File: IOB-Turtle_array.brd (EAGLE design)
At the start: 106.7 x 104.1 mm, 92 parts

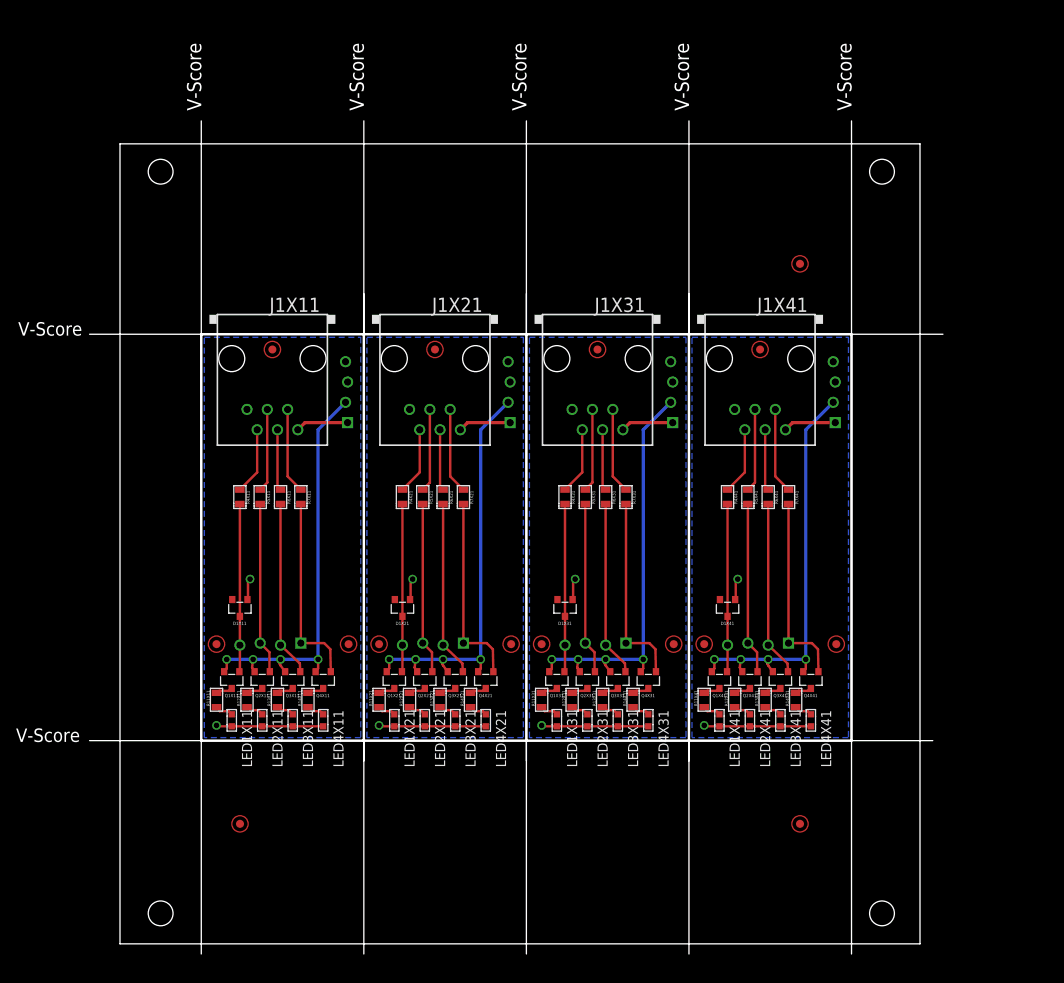
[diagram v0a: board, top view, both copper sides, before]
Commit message: Version 2.0
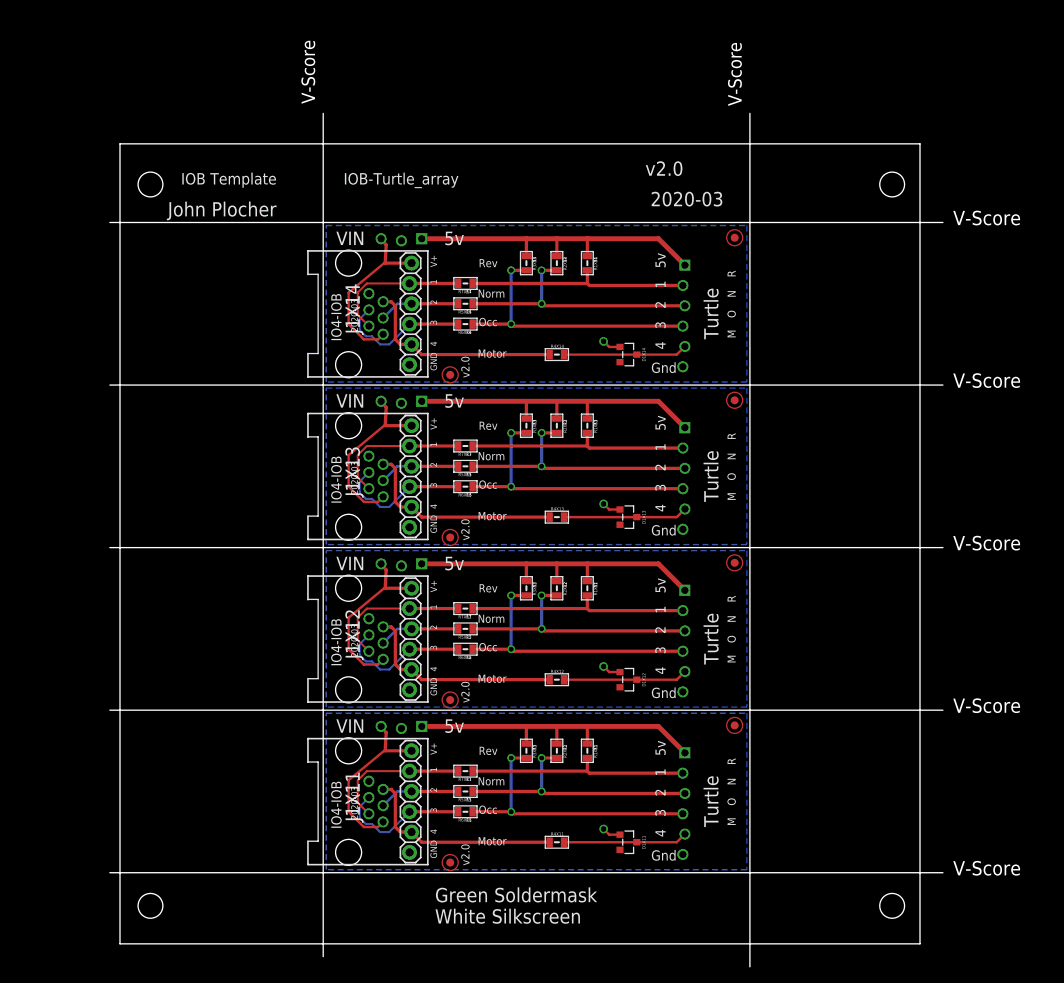
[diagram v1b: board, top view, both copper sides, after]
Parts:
- removed D1X21, D1X31, D1X41, Q1X11, Q1X21, Q1X31, Q1X41, Q2X11, Q2X21, Q2X31, Q2X41, Q3X11, Q3X21, Q3X31, Q3X41, Q4X11, Q4X21, Q4X31, Q4X41: (no value), SPCoast:SOT23-3
- removed FID1X21, FID1X31, FID1X41, FID2X21, FID2X31, FID2X41, FID3X11, FID3X21, FID3X31, FID3X41, R8X2, R8X3, R8X4: (no value), SPCoast:FIDUCIAL_1MM
- removed IOBX11, IOBX21, IOBX31, IOBX41: (no value), SPCoast:IO4-IOB
- removed J1X21, J1X31, J1X41: (no value), SPCoast:RJ25
- removed LED1X11, LED1X21, LED1X31, LED1X41, LED2X11, LED2X21, LED2X31, LED2X41, LED3X11, LED3X21, LED3X31, LED3X41, LED4X11, LED4X21, LED4X31, LED4X41: (no value), SPCoast:0603-LED
- removed R11X11, R11X21, R11X31, R11X41, R12X11, R12X21, R12X31, R12X41, R13X11, R13X21, R13X31, R13X41, R14X11, R14X21, R14X31, R14X41, R4X21, R4X31, R4X41, R5X21, R5X31, R5X41, R6X21, R6X31, R6X41, R7X21, R7X31, R7X41: (no value), SPCoast:0805-RES
- removed R8X1: (no value), SPCoast:BOARD-DINRAIL-3.17IN-4X-IOB
- added D1X12, D1X13, D1X14: (no value), SPCoast:SOT23-3
- added FID1X12, FID1X13, FID1X14, FID2X12, FID2X13, FID2X14: (no value), SPCoast:FIDUCIAL_1MM
- added J1X12, J1X13, J1X14: (no value), SPCoast:RJ24-INVERTED-PINS
- added R1X11, R1X12, R1X13, R1X14, R2X11, R2X12, R2X13, R2X14, R3X11, R3X12, R3X13, R3X14, R4X12, R4X13, R4X14, R5X12, R5X13, R5X14, R6X12, R6X13, R6X14, R7X12, R7X13, R7X14: (no value), SPCoast:0805-RES
- added U$1X1: (no value), SPCoast:BOARD-DINRAIL-3.17IN-H4X-IOB
- added U$1X11, U$1X12, U$1X13, U$1X14: (no value), SPCoast:IO4-IOB
- J1X11: device SPCoast:RJ25 -> SPCoast:RJ24-INVERTED-PINS
- moved FID1X11 67.9 mm to (41.3, 10.2), turned to 0 degrees
- moved FID2X11 65.6 mm to (76.8, 27.3), turned to 0 degrees
- moved R4X11 58.6 mm to (54.6, 12.7), turned to 0 degrees
- moved J1X11 57.0 mm to (32.4, 17.8), turned to 90 degrees
- moved D1X11 56.7 mm to (63.5, 12.7), turned to 270 degrees
- moved R6X11 45.7 mm to (43.2, 16.5), turned to 180 degrees
- moved R5X11 44.9 mm to (43.2, 19.1), turned to 180 degrees
- moved R7X11 40.0 mm to (43.2, 21.6), turned to 180 degrees
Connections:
- removed net !KTX11: J1X11.5, R4X11.1
- removed net !KTX21: J1X21.5, R4X21.1
- removed net !KTX31: J1X31.5, R4X31.1
- removed net !KTX41: J1X41.5, R4X41.1
- removed net !NORMX21: J1X21.3, R6X21.1
- removed net !NORMX31: J1X31.3, R6X31.1
- removed net !NORMX41: J1X41.3, R6X41.1
- removed net !OCCX21: J1X21.4, R5X21.1
- removed net !OCCX31: J1X31.4, R5X31.1
- removed net !OCCX41: J1X41.4, R5X41.1
- removed net !REVX21: J1X21.2, R7X21.1
- removed net !REVX31: J1X31.2, R7X31.1
- removed net !REVX41: J1X41.2, R7X41.1
- removed net GNDX21: D1X21.1, IOBX21.G@1, IOBX21.G@2, J1X21.6, LED1X21.C, LED2X21.C, LED3X21.C, LED4X21.C
- removed net GNDX31: D1X31.1, IOBX31.G@1, IOBX31.G@2, J1X31.6, LED1X31.C, LED2X31.C, LED3X31.C, LED4X31.C
- removed net GNDX41: D1X41.1, IOBX41.G@1, IOBX41.G@2, J1X41.6, LED1X41.C, LED2X41.C, LED3X41.C, LED4X41.C
- removed net N$11X11: Q4X11.3, R14X11.2
- removed net N$11X21: Q4X21.3, R14X21.2
- removed net N$11X31: Q4X31.3, R14X31.2
- removed net N$11X41: Q4X41.3, R14X41.2
- removed net N$2X11: LED4X11.A, R14X11.1
- removed net N$2X21: LED4X21.A, R14X21.1
- removed net N$2X31: LED4X31.A, R14X31.1
- removed net N$2X41: LED4X41.A, R14X41.1
- removed net N$30X11: Q3X11.3, R13X11.2
- removed net N$30X21: Q3X21.3, R13X21.2
- removed net N$30X31: Q3X31.3, R13X31.2
- removed net N$30X41: Q3X41.3, R13X41.2
- removed net N$31X11: Q2X11.3, R12X11.2
- removed net N$31X21: Q2X21.3, R12X21.2
- removed net N$31X31: Q2X31.3, R12X31.2
- removed net N$31X41: Q2X41.3, R12X41.2
- removed net N$32X11: Q1X11.3, R11X11.2
- removed net N$32X21: Q1X21.3, R11X21.2
- removed net N$32X31: Q1X31.3, R11X31.2
- removed net N$32X41: Q1X41.3, R11X41.2
- removed net N$3X11: LED3X11.A, R13X11.1
- removed net N$3X21: LED3X21.A, R13X21.1
- removed net N$3X31: LED3X31.A, R13X31.1
- removed net N$3X41: LED3X41.A, R13X41.1
- removed net N$4X11: LED2X11.A, R12X11.1
- removed net N$4X21: LED2X21.A, R12X21.1
- removed net N$4X31: LED2X31.A, R12X31.1
- removed net N$4X41: LED2X41.A, R12X41.1
- removed net N$5X11: LED1X11.A, R11X11.1
- removed net N$5X21: LED1X21.A, R11X21.1
- removed net N$5X31: LED1X31.A, R11X31.1
- removed net N$5X41: LED1X41.A, R11X41.1
- removed net P1X11: IOBX11.P1, Q4X11.1, R7X11.2
- removed net P1X21: IOBX21.P1, Q4X21.1, R7X21.2
- removed net P1X31: IOBX31.P1, Q4X31.1, R7X31.2
- removed net P1X41: IOBX41.P1, Q4X41.1, R7X41.2
- removed net P2X11: IOBX11.P2, Q3X11.1, R6X11.2
- removed net P2X21: IOBX21.P2, Q3X21.1, R6X21.2
- removed net P2X31: IOBX31.P2, Q3X31.1, R6X31.2
- removed net P2X41: IOBX41.P2, Q3X41.1, R6X41.2
- removed net P3X11: IOBX11.P3, Q2X11.1, R5X11.2
- removed net P3X21: IOBX21.P3, Q2X21.1, R5X21.2
- removed net P3X31: IOBX31.P3, Q2X31.1, R5X31.2
- removed net P3X41: IOBX41.P3, Q2X41.1, R5X41.2
- removed net P4X21: D1X21.3, IOBX21.P4, Q1X21.1, R4X21.2
- removed net P4X31: D1X31.3, IOBX31.P4, Q1X31.1, R4X31.2
- removed net P4X41: D1X41.3, IOBX41.P4, Q1X41.1, R4X41.2
- removed net VCCIOX21: IOBX21.V+, J1X21.1
- removed net VCCIOX31: IOBX31.V+, J1X31.1
- removed net VCCIOX41: IOBX41.V+, J1X41.1
- removed net VCCX21: IOBX21.V5, Q1X21.2, Q2X21.2, Q3X21.2, Q4X21.2
- removed net VCCX31: IOBX31.V5, Q1X31.2, Q2X31.2, Q3X31.2, Q4X31.2
- removed net VCCX41: IOBX41.V5, Q1X41.2, Q2X41.2, Q3X41.2, Q4X41.2
- new net !NORMX12: R2X12.2, R5X12.1, U$1X12.P2
- new net !NORMX13: R2X13.2, R5X13.1, U$1X13.P2
- new net !NORMX14: R2X14.2, R5X14.1, U$1X14.P2
- new net !OCCX12: R3X12.2, R6X12.1, U$1X12.P3
- new net !OCCX13: R3X13.2, R6X13.1, U$1X13.P3
- new net !OCCX14: R3X14.2, R6X14.1, U$1X14.P3
- new net !REVX12: R1X12.2, R7X12.1, U$1X12.P1
- new net !REVX13: R1X13.2, R7X13.1, U$1X13.P1
- new net !REVX14: R1X14.2, R7X14.1, U$1X14.P1
- new net GNDX12: D1X12.1, J1X12.6, J1X12.6@1, U$1X12.G@3
- new net GNDX13: D1X13.1, J1X13.6, J1X13.6@1, U$1X13.G@3
- new net GNDX14: D1X14.1, J1X14.6, J1X14.6@1, U$1X14.G@3
- new net IO4-2X11: J1X11.2, J1X11.2@1, R7X11.2
- new net IO4-2X12: J1X12.2, J1X12.2@1, R7X12.2
- new net IO4-2X13: J1X13.2, J1X13.2@1, R7X13.2
- new net IO4-2X14: J1X14.2, J1X14.2@1, R7X14.2
- new net IO4-3X11: J1X11.3, J1X11.3@1, R5X11.2
- new net IO4-3X12: J1X12.3, J1X12.3@1, R5X12.2
- new net IO4-3X13: J1X13.3, J1X13.3@1, R5X13.2
- new net IO4-3X14: J1X14.3, J1X14.3@1, R5X14.2
- new net IO4-4X11: J1X11.4, J1X11.4@1, R6X11.2
- new net IO4-4X12: J1X12.4, J1X12.4@1, R6X12.2
- new net IO4-4X13: J1X13.4, J1X13.4@1, R6X13.2
- new net IO4-4X14: J1X14.4, J1X14.4@1, R6X14.2
- new net IO4-5X11: J1X11.5, J1X11.5@1, R4X11.1
- new net IO4-5X12: J1X12.5, J1X12.5@1, R4X12.1
- new net IO4-5X13: J1X13.5, J1X13.5@1, R4X13.1
- new net IO4-5X14: J1X14.5, J1X14.5@1, R4X14.1
- new net P4X12: D1X12.3, R4X12.2, U$1X12.P4
- new net P4X13: D1X13.3, R4X13.2, U$1X13.P4
- new net P4X14: D1X14.3, R4X14.2, U$1X14.P4
- new net VCCIOX12: J1X12.1, J1X12.1@1, U$1X12.V+
- new net VCCIOX13: J1X13.1, J1X13.1@1, U$1X13.V+
- new net VCCIOX14: J1X14.1, J1X14.1@1, U$1X14.V+
- new net VCCX12: R1X12.1, R2X12.1, R3X12.1, U$1X12.V5, U$1X12.V5@1
- new net VCCX13: R1X13.1, R2X13.1, R3X13.1, U$1X13.V5, U$1X13.V5@1
- new net VCCX14: R1X14.1, R2X14.1, R3X14.1, U$1X14.V5, U$1X14.V5@1
- net !NORMX11: now also R2X11.2, R5X11.1, U$1X11.P2; no longer J1X11.3, R6X11.1
- net !OCCX11: now also R3X11.2, R6X11.1, U$1X11.P3; no longer J1X11.4, R5X11.1
- net !REVX11: now also R1X11.2, U$1X11.P1; no longer J1X11.2
- net GNDX11: now also J1X11.6@1, U$1X11.G@3; no longer IOBX11.G@1, IOBX11.G@2, LED1X11.C, LED2X11.C, LED3X11.C, LED4X11.C
- net P4X11: now also U$1X11.P4; no longer IOBX11.P4, Q1X11.1
- net VCCIOX11: now also J1X11.1@1, U$1X11.V+; no longer IOBX11.V+
- net VCCX11: now also R1X11.1, R2X11.1, R3X11.1, U$1X11.V5, U$1X11.V5@1; no longer IOBX11.V5, Q1X11.2, Q2X11.2, Q3X11.2, Q4X11.2
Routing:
- net VCCX31: track 51.7 -> 0.00 mm, vias 4 -> 0
- net VCCX21: track 51.7 -> 0.00 mm, vias 4 -> 0
- net VCCX41: track 51.7 -> 0.00 mm, vias 4 -> 0
- net VCCX14: track 0.00 -> 40.7 mm
- net VCCX13: track 0.00 -> 40.7 mm
- net VCCX12: track 0.00 -> 40.7 mm
- net !OCCX14: track 0.00 -> 35.0 mm, vias 0 -> 2
- net !OCCX13: track 0.00 -> 35.0 mm, vias 0 -> 2
- net !OCCX12: track 0.00 -> 35.0 mm, vias 0 -> 2
- net !NORMX13: track 0.00 -> 32.7 mm, vias 0 -> 2
- net !NORMX12: track 0.00 -> 32.7 mm, vias 0 -> 2
- net !NORMX14: track 0.00 -> 32.7 mm, vias 0 -> 2
- net !REVX13: track 0.00 -> 28.0 mm
- net !REVX12: track 0.00 -> 28.0 mm
- net !REVX14: track 0.00 -> 28.0 mm
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- added copper zone on layer 16, net GNDX12
- added copper zone on layer 16, net GNDX13
- added copper zone on layer 16, net GNDX14
- removed copper zone on layer 16, net GNDX21
- removed copper zone on layer 16, net GNDX31
- removed copper zone on layer 16, net GNDX41
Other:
- board size 106.7 x 104.1 mm -> 104.1 x 106.7 mm
- board text added: "2020-03"
- board text added: "D1"
- board text added: "Green Soldermask White Silkscreen"
- board text added: "J1"
- board text added: "R1"
- board text added: "R2"
- board text added: "R3"
- board text added: "R4"
- board text added: "R5"
- board text added: "R6"
- board text added: "R7"
- board text added: "v2.0"
- board text removed: "(15,15)"
- board text removed: "(15,85)"
- board text removed: "(85,85)"
- board text removed: "2018-02"
- board text removed: "Green Soldermask, White Silkscreen"
- board text removed: "IO Interface"
- board text removed: "IOB Turtle"
- board text removed: "Made in the PCR, Coast Div, NMRA"
- board text removed: "Model Railroading is Fun!"
- board text removed: "V1.1"
- board text removed: "v1.1"
